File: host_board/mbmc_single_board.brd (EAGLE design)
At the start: 116.5 x 81.3 mm, 114 parts, among them IC1 ULN2803, IC15 PIC18F57K42-E_PT, IC16 REF3440IDBVR, IC17 MAX232, IC2 DIP Socket, IC3 REF02 5 VOLTS, IC4 5 VOLTS, IC5 12 VOLTS, IC6 3.3 VOLTS, J1 1-1586043-4, J2 1586044-4, Q3 ASF1, X15 RX-2, X16 TX-2, X17 RESETJMP

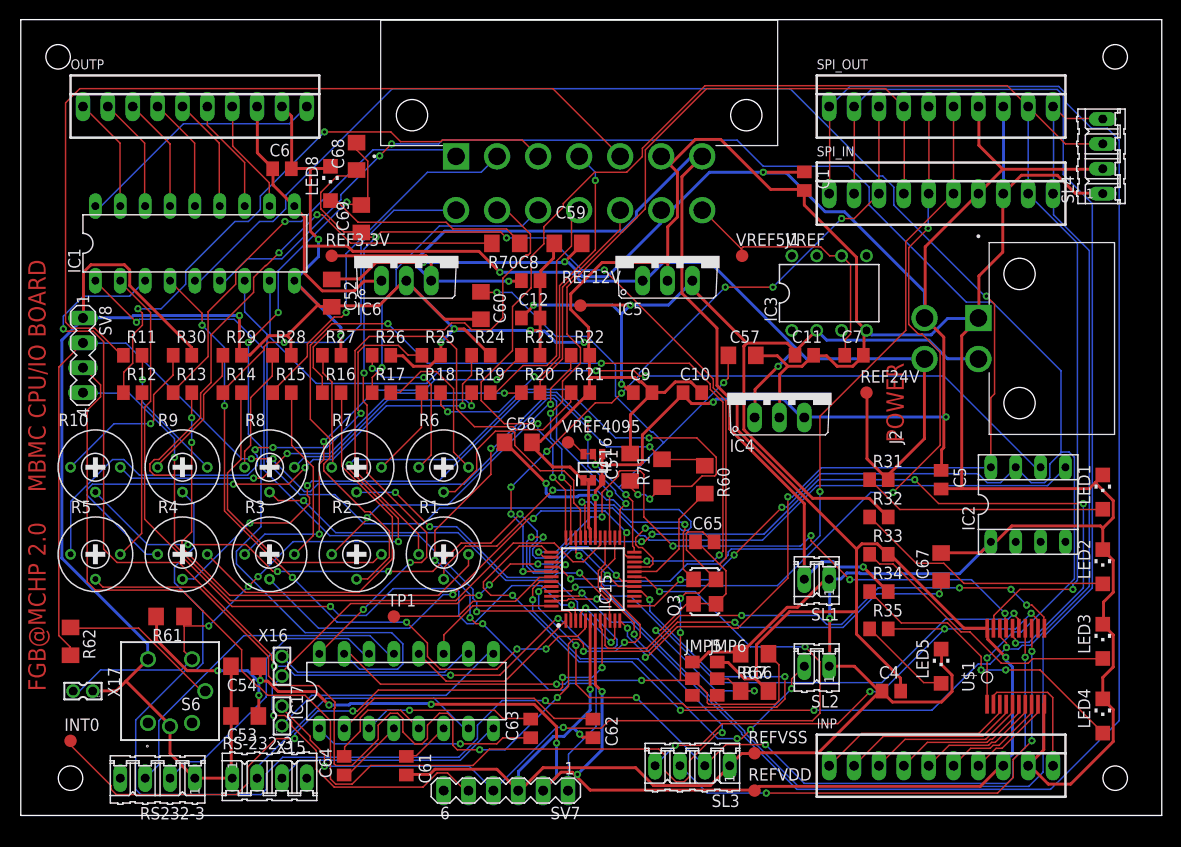
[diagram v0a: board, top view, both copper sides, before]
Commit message: up
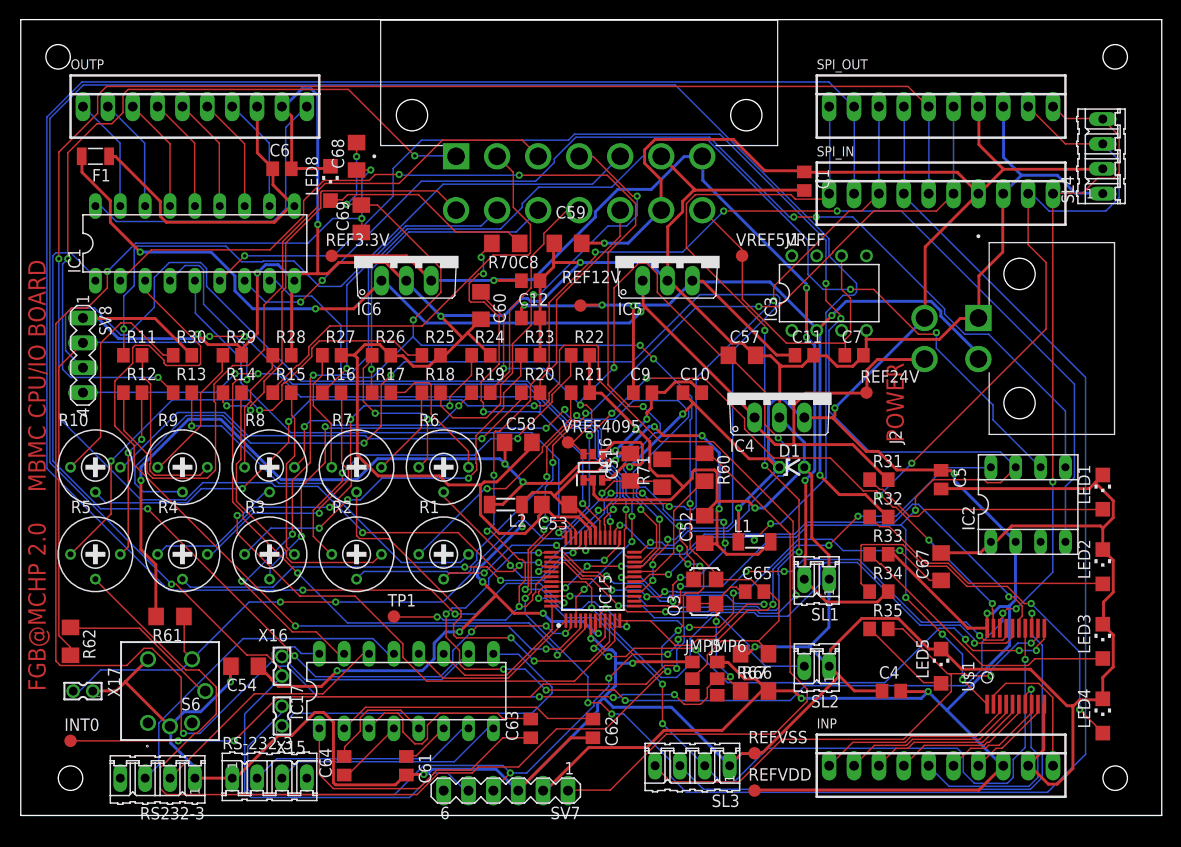
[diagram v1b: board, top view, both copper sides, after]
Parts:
- added D1: 5.6v, diode:ZDIO-2.5
- added F1: 1206L050, polyfuse-smd_10:1206L
- added L1, L2: 1000, inductor-neosid:SM-1206
- moved C52 45.1 mm to (69.8, 29.2), turned to 90 degrees
- moved C53 38.4 mm to (54.6, 31.8)
- moved C65 7.18 mm to (74.9, 22.9)
- moved R60 1.27 mm to (69.8, 35.6)
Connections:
- new net N$21: C6.1, F1.1, IC1.10, OUTP.8
- new net N$22: C52.1, C53.1, C54.1, IC15.30, IC15.7, L1.2, L2.1
- net +24V: now also F1.2; no longer C6.1, IC1.10, OUTP.8
- net N$255: now also IC2.4
- net VDD: now also D1.C, IC2.2, L1.1, L2.2; no longer C52.1, C53.1, C54.1, IC15.30, IC15.7
- net VSS: now also D1.A
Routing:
- net N$233: track 73.3 -> 245.7 mm, vias 5 -> 4
- net N$255: track 17.8 -> 136.6 mm, vias 0 -> 7
- net N$260: track 83.4 -> 188.5 mm, vias 3 -> 4
- net N$22: track 0.00 -> 104.2 mm, vias 0 -> 10
- net N$67: track 170.9 -> 95.5 mm, vias 1 -> 4
- net N$259: track 84.3 -> 155.4 mm, vias 2 -> 3
- net N$282: track 68.7 -> 121.4 mm
- net N$283: track 170.7 -> 124.7 mm, vias 4 -> 6
- net N$251: track 133.6 -> 87.6 mm, vias 2 -> 1
- net N$74: track 43.0 -> 80.8 mm, vias 1 -> 3
- net VSS: track 658.2 -> 695.4 mm, vias 10 -> 14
- net N$265: track 101.5 -> 65.3 mm, vias 4 -> 3
- net N$252: track 127.9 -> 92.4 mm, vias 3 -> 6
- net N$277: track 93.0 -> 57.9 mm, vias 8 -> 2
- net N$21: track 0.00 -> 35.1 mm
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
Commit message: up
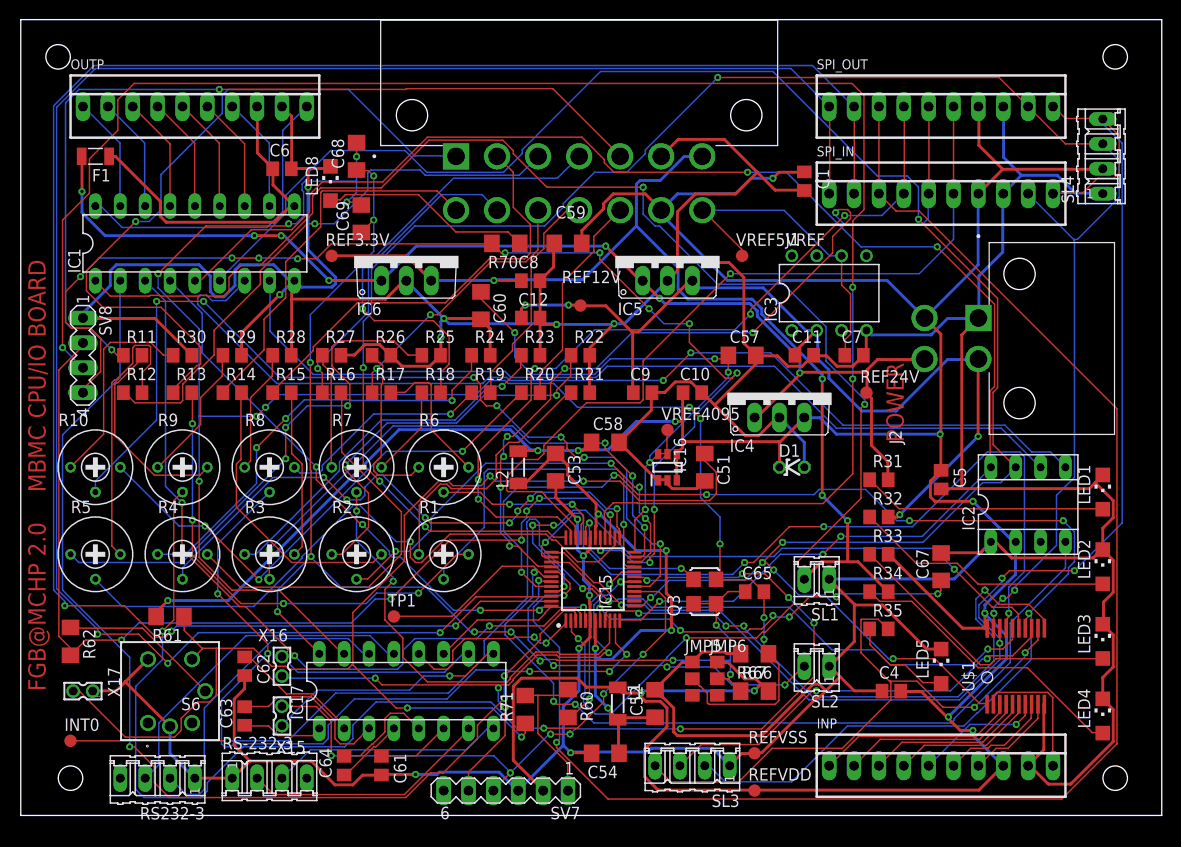
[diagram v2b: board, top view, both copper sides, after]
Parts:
- moved C54 37.9 mm to (59.7, 6.35)
- moved C62 36.1 mm to (22.9, 15.2)
- moved C63 29.2 mm to (22.9, 10.2)
- moved R60 27.9 mm to (55.9, 11.4)
- moved R71 27.9 mm to (51.5, 10.8)
- moved L1 21.6 mm to (61.0, 11.4), turned to 270 degrees
- moved C52 18.5 mm to (64.8, 11.4)
- moved VREF4095 10.2 mm to (66.0, 39.4)
- moved C58 8.89 mm to (59.7, 38.1)
- moved IC16 7.62 mm to (66.0, 35.6)
- moved C51 7.62 mm to (69.8, 35.6), turned to 270 degrees
- moved L2 4.02 mm to (50.8, 35.6), turned to 90 degrees
- moved C53 3.81 mm to (54.6, 35.6), turned to 270 degrees
- moved C61 2.54 mm to (36.8, 5.08)
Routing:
- net N$233: track 245.7 -> 58.7 mm, vias 4 -> 5
- net N$67: track 95.5 -> 197.1 mm, vias 4 -> 3
- net N$260: track 188.5 -> 87.6 mm, vias 4 -> 7
- net N$258: track 70.1 -> 161.3 mm, vias 4 -> 2
- net N$251: track 87.6 -> 176.8 mm, vias 1 -> 3
- net N$259: track 155.4 -> 81.5 mm, vias 3 -> 5
- net N$272: track 93.1 -> 162.1 mm, vias 5 -> 4
- net VCC: track 185.3 -> 123.0 mm, vias 9 -> 11
- net N$39: track 133.4 -> 192.7 mm, vias 8 -> 7
- net N$270: track 80.8 -> 129.9 mm, vias 4 -> 6
- net N$299: track 76.1 -> 125.0 mm, vias 3 -> 4
- net N$300: track 62.8 -> 15.6 mm
- net N$262: track 112.6 -> 65.8 mm, vias 6 -> 1
- net N$22: track 104.2 -> 60.1 mm, vias 10 -> 5
- net VSS: track 695.4 -> 658.2 mm, vias 14 -> 12
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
